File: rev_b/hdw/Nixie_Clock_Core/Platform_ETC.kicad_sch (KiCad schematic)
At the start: 7 parts

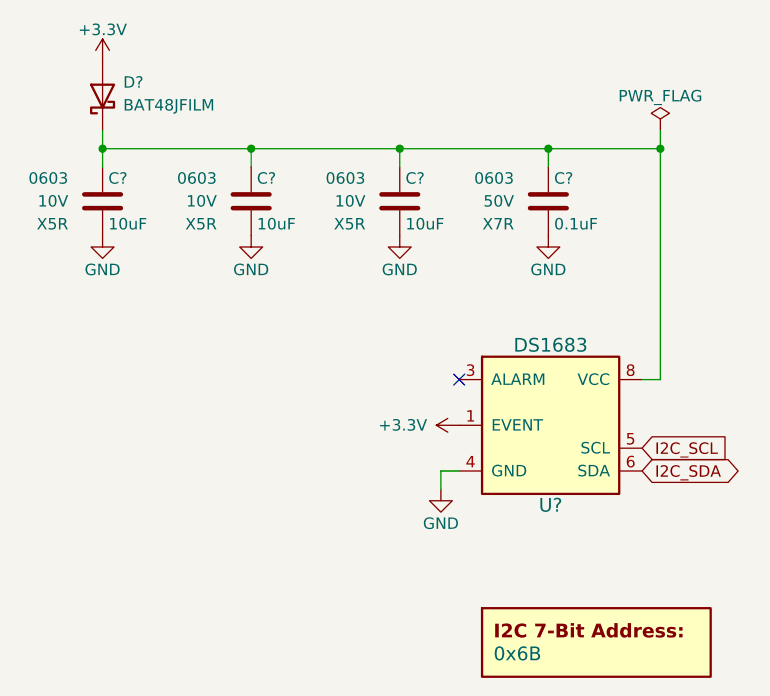
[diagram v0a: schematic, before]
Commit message: more rev b sch progress
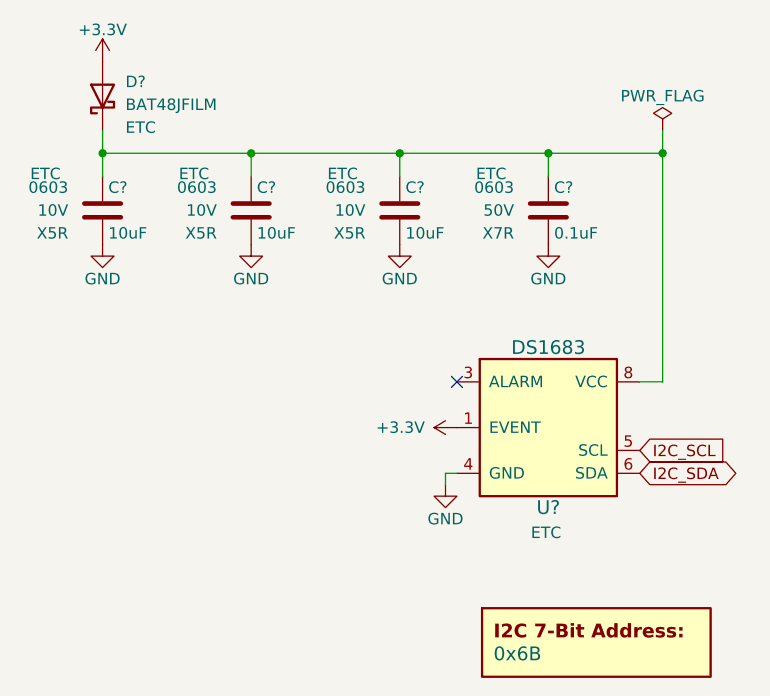
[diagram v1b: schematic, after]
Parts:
- removed C? (x2): 10uF, Capacitors_SMD:C_0603, symbol Custom_Library:C_Custom
- added C? (x2): 10uF, Capacitors_SMD:C_0603, symbol Custom_Library:C_Custom
- C? (x2), D?: Configuration (none) -> ETC
- U?: Config TOF -> ETC
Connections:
- net GND: now also C?.2, C?.2
- net at C?.1, C?.1, D?.1 (K)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: now also C?.1, C?.1
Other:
- moved on the sheet: C?
